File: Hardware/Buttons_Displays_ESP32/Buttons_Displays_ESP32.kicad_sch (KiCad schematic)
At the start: 24 parts, among them J1 Conn_01x09, J2 Conn_01x09, J3 Conn_01x09, J4 Conn_01x09, J5 i2c, J6 USB_C_Receptacle_USB2.0_16P, SW1 SW_Push, SW2 SW_Push, U1 ESP32-S3-WROOM-1, U2 USBLC6-2P6

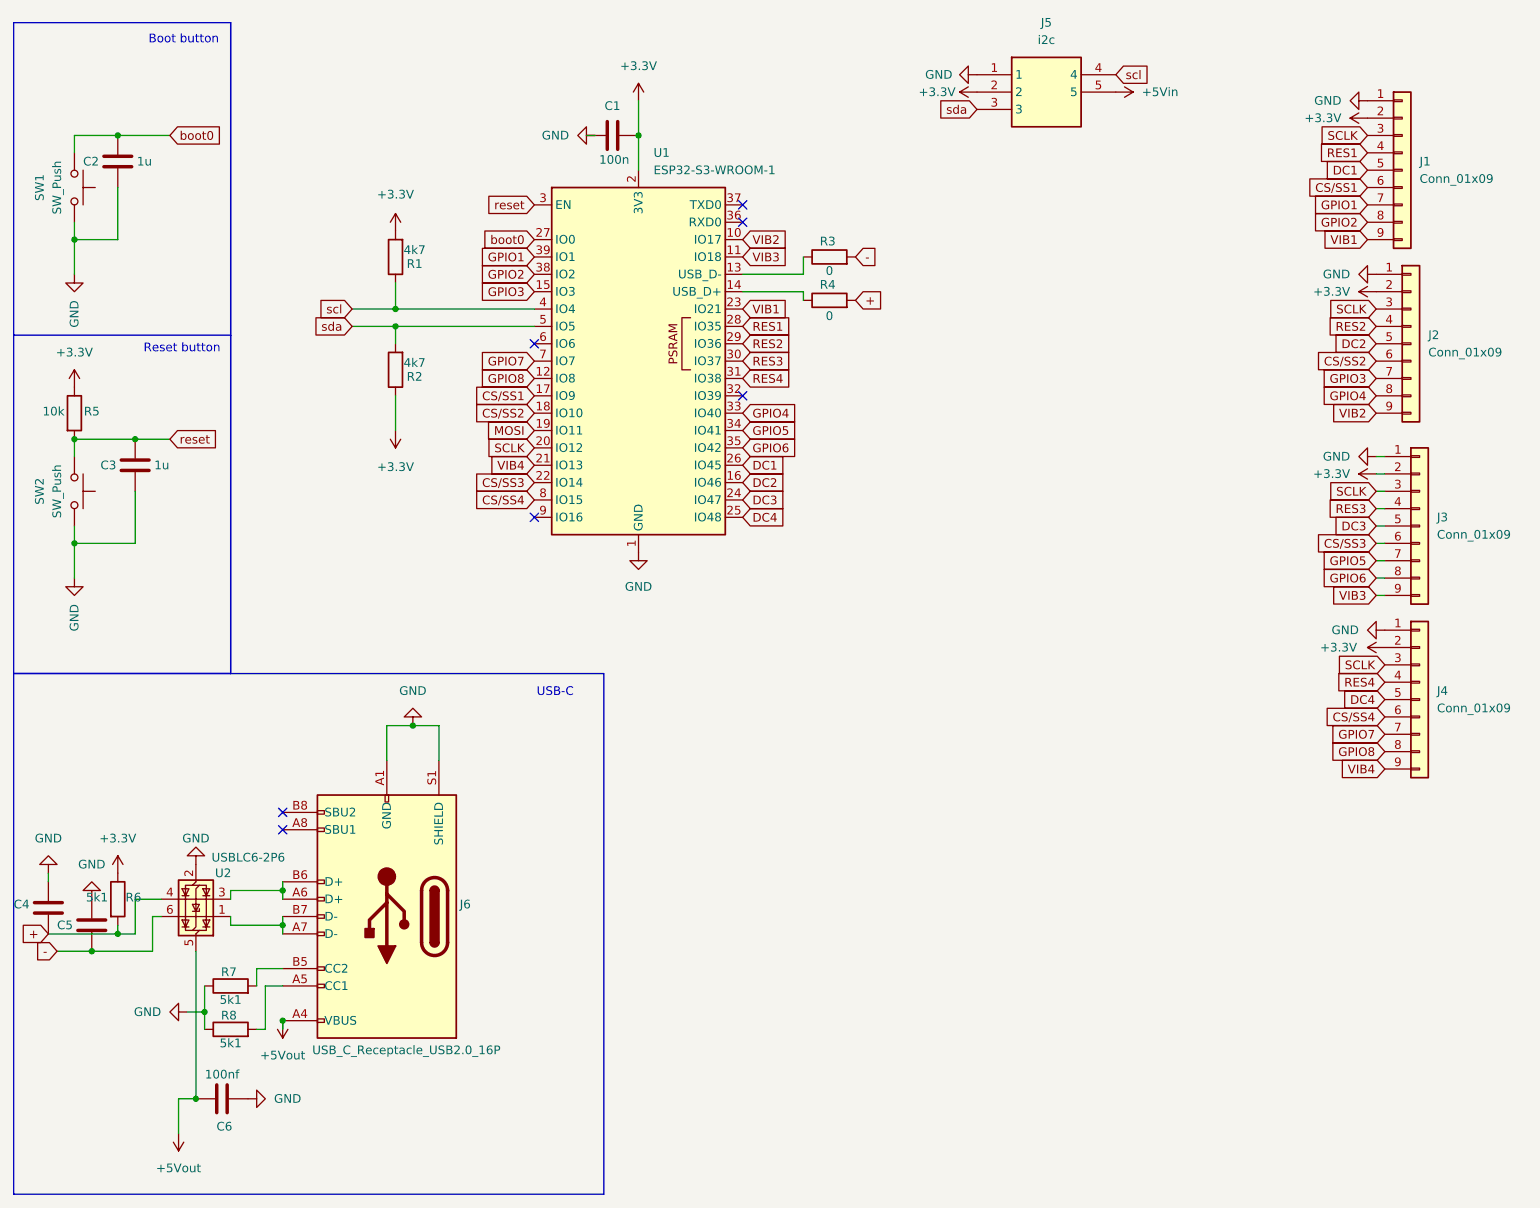
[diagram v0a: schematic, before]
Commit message: laatste aanpassingen
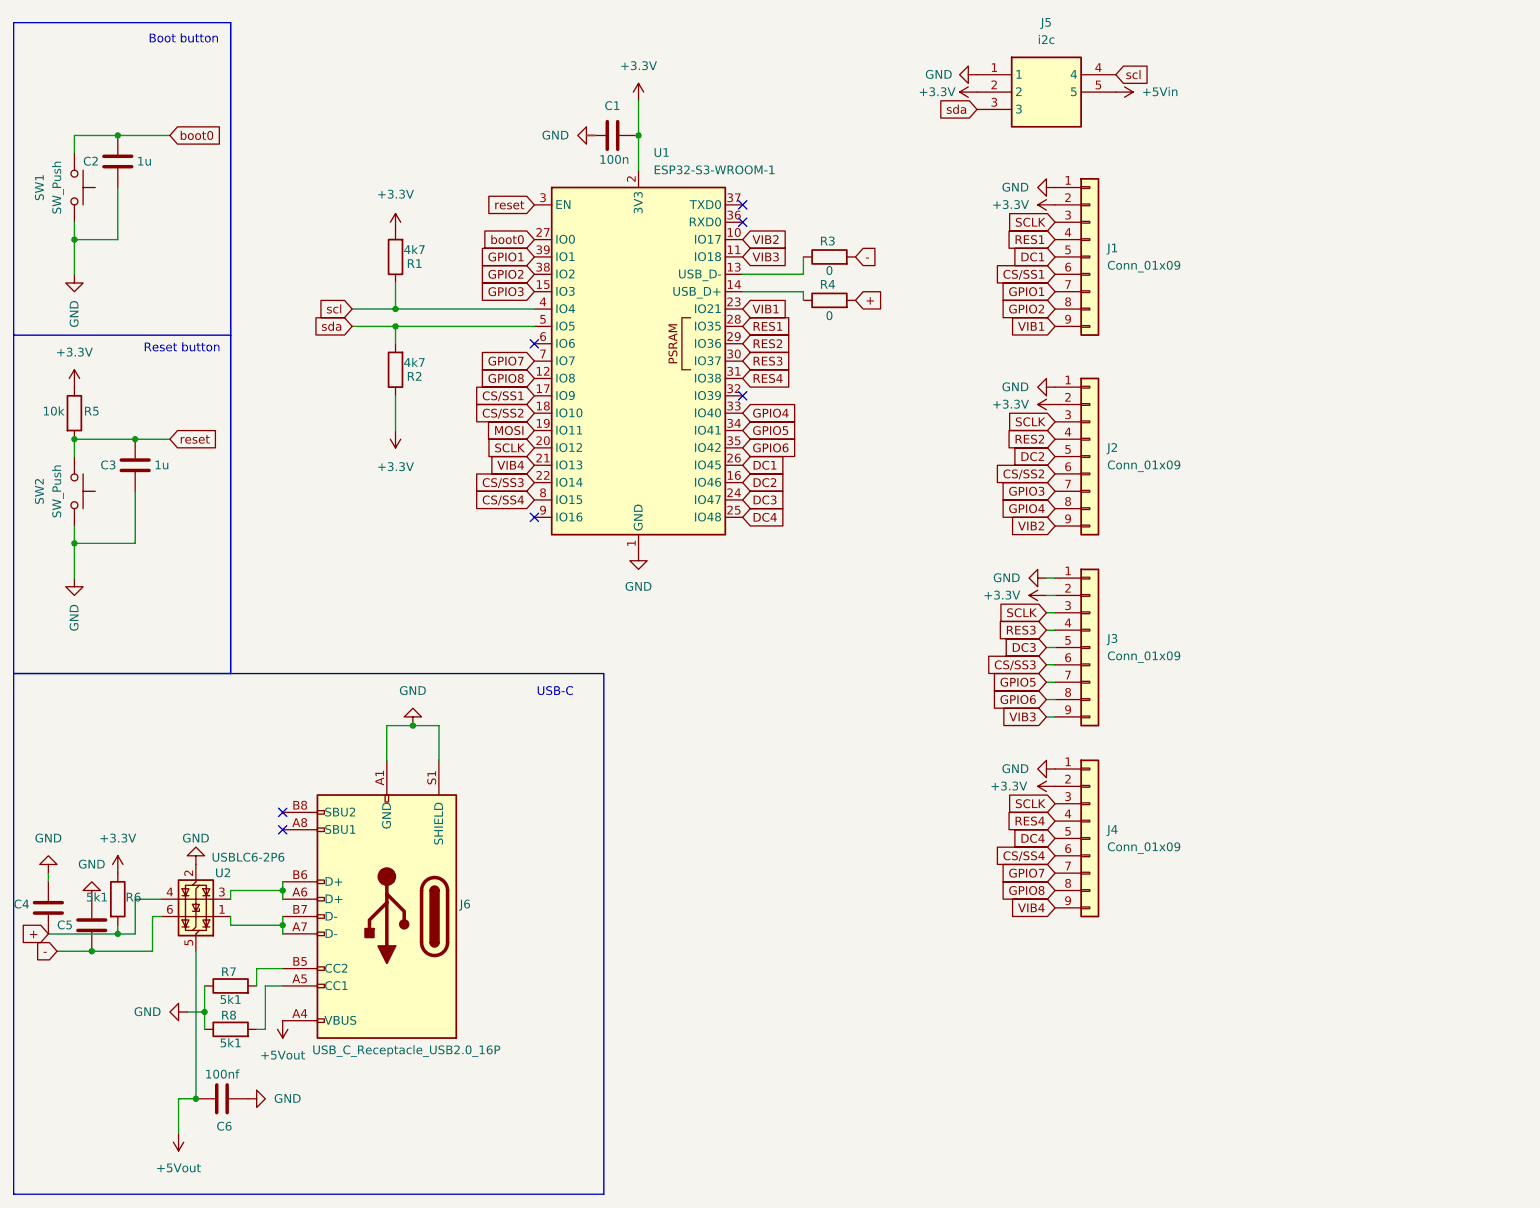
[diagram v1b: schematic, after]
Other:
- moved on the sheet: J1, J2, J3, J4
